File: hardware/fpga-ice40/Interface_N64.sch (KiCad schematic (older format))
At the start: 7 parts, among them J6 Conn_02x20_Odd_Even

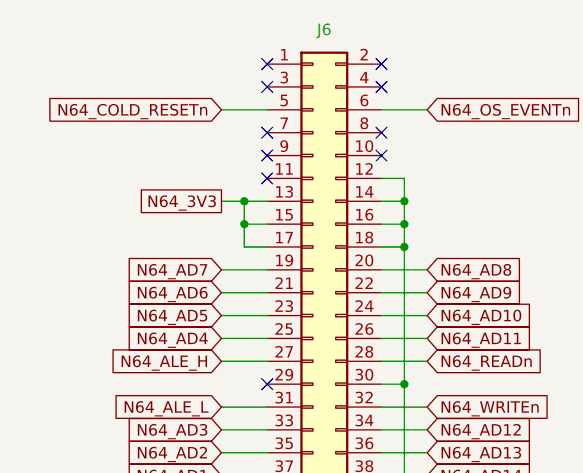
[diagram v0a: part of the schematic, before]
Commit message: Completed verification of all pins for all symbols
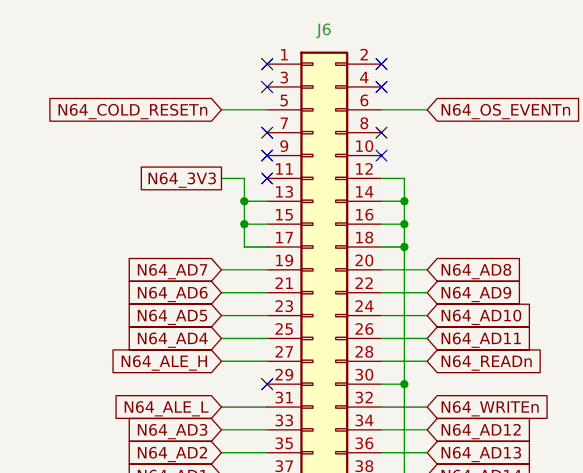
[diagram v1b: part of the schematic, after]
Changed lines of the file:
@@
 	3200 4100 3200 4000
 Wire Wire Line
-	3200 4000 3100 4000
-Connection ~ 3200 4000
+	3200 3900 3100 3900
 NoConn ~ 3300 3400
 NoConn ~ 3300 3500
@@
 Text GLabel 4000 5300 2    50   Input ~ 0
 N64_AD15
-Text GLabel 3100 4000 0    50   UnSpc ~ 0
+Text GLabel 3100 3900 0    50   UnSpc ~ 0
 N64_3V3
 $Comp
@@
 Text GLabel 7950 4500 2    50   Input ~ 0
 N64_AD7_IC
+Wire Wire Line
+	3200 3900 3200 4000
+Connection ~ 3200 4000
 $EndSCHEMATC
